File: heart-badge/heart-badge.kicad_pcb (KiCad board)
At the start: 2 copper layers, 37 x 32.6 mm, 18 parts

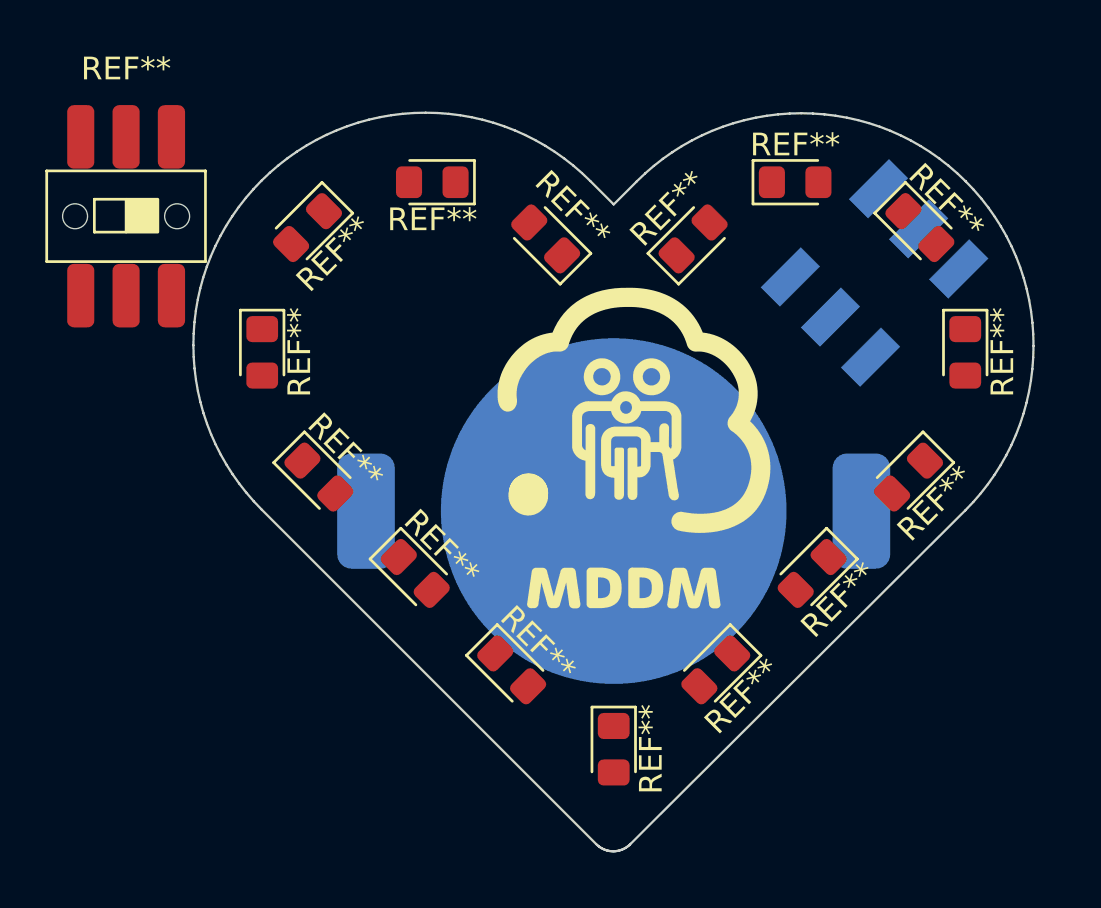
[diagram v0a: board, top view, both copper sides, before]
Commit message: another one
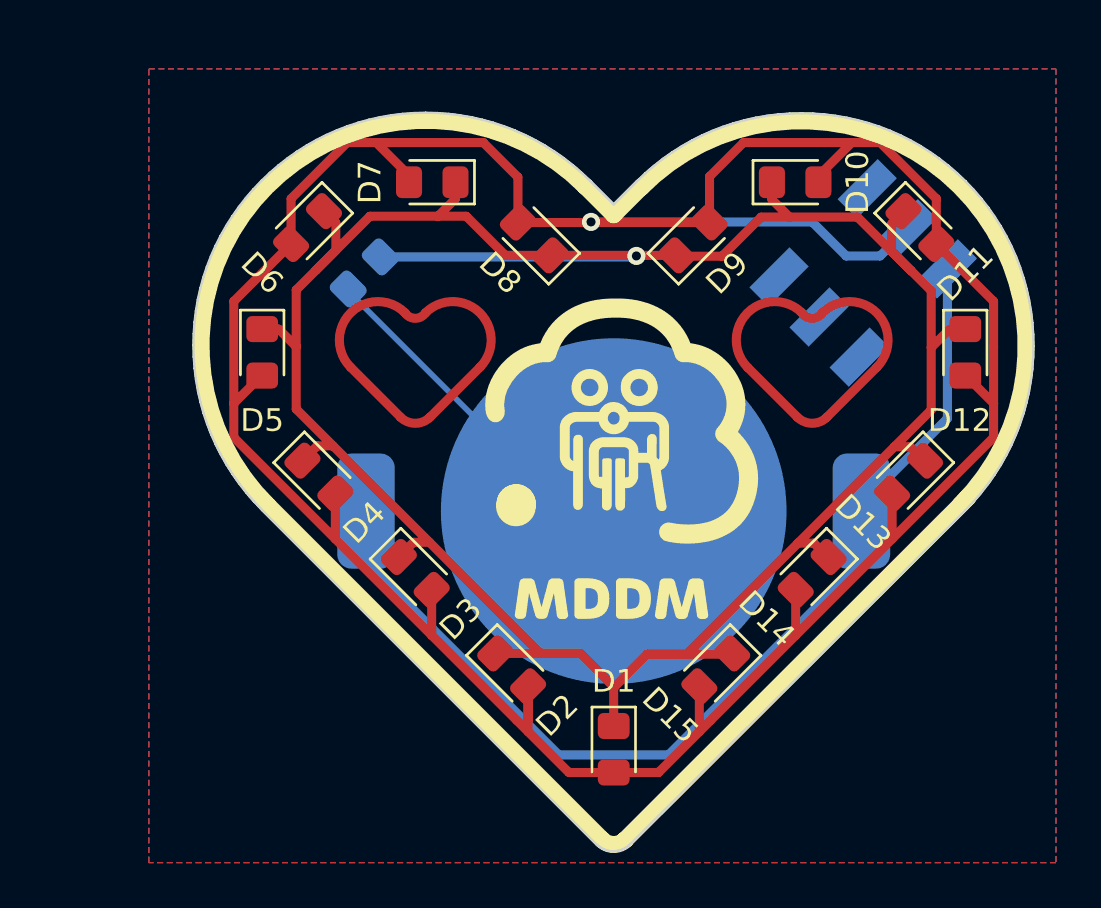
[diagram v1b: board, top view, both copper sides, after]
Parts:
- removed REF** (x15): LED_0805_2012Metric_Pad1.15x1.40mm_HandSolder, LED_SMD:LED_0805_2012Metric_Pad1.15x1.40mm_HandSolder
- removed REF**: CR2032_SMD, lib:CR2032_SMD
- removed REF**: SW_JS202011SCQN, lib:SW_JS202011SCQN
- removed REF**: MS-22D28-G020, lib:MS-22D28-G020
- added BT1: Battery_Cell, lib:CR2032_SMD, B.Cu at (143.0, 77.0)
- added D1: LED, LED_SMD:LED_0805_2012Metric_Pad1.15x1.40mm_HandSolder, F.Cu at (143.0, 87.5)
- added D10: LED, LED_SMD:LED_0805_2012Metric_Pad1.15x1.40mm_HandSolder, F.Cu at (151.0, 62.5)
- added D11: LED, LED_SMD:LED_0805_2012Metric_Pad1.15x1.40mm_HandSolder, F.Cu at (156.5, 64.5)
- added D12: LED, LED_SMD:LED_0805_2012Metric_Pad1.15x1.40mm_HandSolder, F.Cu at (158.5, 70.0)
- added D13: LED, LED_SMD:LED_0805_2012Metric_Pad1.15x1.40mm_HandSolder, F.Cu at (156.0, 75.5)
- added D14: LED, LED_SMD:LED_0805_2012Metric_Pad1.15x1.40mm_HandSolder, F.Cu at (151.8, 79.8)
- added D15: LED, LED_SMD:LED_0805_2012Metric_Pad1.15x1.40mm_HandSolder, F.Cu at (147.5, 84.0)
- added D2: LED, LED_SMD:LED_0805_2012Metric_Pad1.15x1.40mm_HandSolder, F.Cu at (138.5, 84.0)
- added D3: LED, LED_SMD:LED_0805_2012Metric_Pad1.15x1.40mm_HandSolder, F.Cu at (134.2, 79.8)
- added D4: LED, LED_SMD:LED_0805_2012Metric_Pad1.15x1.40mm_HandSolder, F.Cu at (130.0, 75.5)
- added D5: LED, LED_SMD:LED_0805_2012Metric_Pad1.15x1.40mm_HandSolder, F.Cu at (127.5, 70.0)
- added D6: LED, LED_SMD:LED_0805_2012Metric_Pad1.15x1.40mm_HandSolder, F.Cu at (129.5, 64.5)
- added D7: LED, LED_SMD:LED_0805_2012Metric_Pad1.15x1.40mm_HandSolder, F.Cu at (135.0, 62.5)
- added D8: LED, LED_SMD:LED_0805_2012Metric_Pad1.15x1.40mm_HandSolder, F.Cu at (139.5, 65.0)
- added D9: LED, LED_SMD:LED_0805_2012Metric_Pad1.15x1.40mm_HandSolder, F.Cu at (146.5, 65.0)
- added R1: 200R, Resistor_SMD:R_0805_2012Metric_Pad1.20x1.40mm_HandSolder, B.Cu at (132.0, 66.5)
- added SW1: MST22D18G2, lib:SW_JS202011SCQN, B.Cu at (154.0, 66.5)
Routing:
- net Net-(D1-A): track 0.00 -> 141.5 mm, vias 0 -> 1
- net Net-(D1-K): track 0.00 -> 120.9 mm, vias 0 -> 1
- net Net-(BT1-+): track 0.00 -> 45.9 mm
- net Net-(BT1--): track 0.00 -> 16.1 mm
- added copper zone on B.Cu, net (none)
- added copper zone on F.Cu, net (none)
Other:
- board text added: "JLCJLCJLCJLC"
- board text added: "github.com/polaracep"
